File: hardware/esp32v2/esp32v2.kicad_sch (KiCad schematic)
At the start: 27 parts, among them J1 Conn_01x02, J2 Conn_01x02, J3 Conn_01x10, U1 ESP32-S3, Y2 40MHz(10ppm)

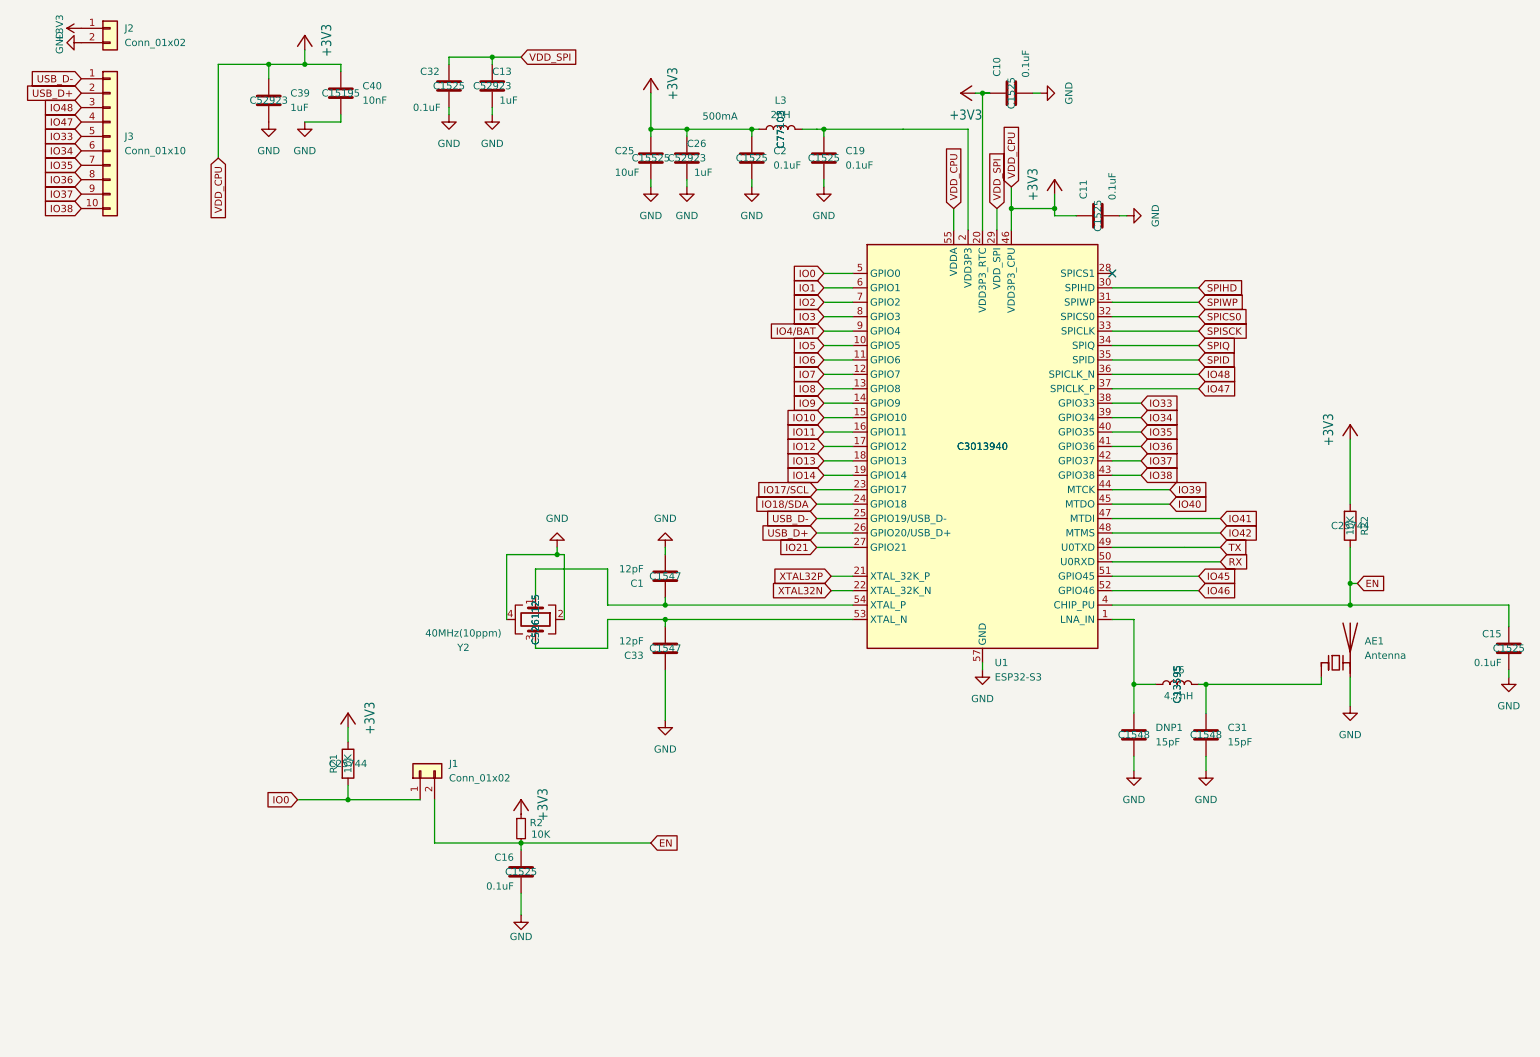
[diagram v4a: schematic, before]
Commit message: wip
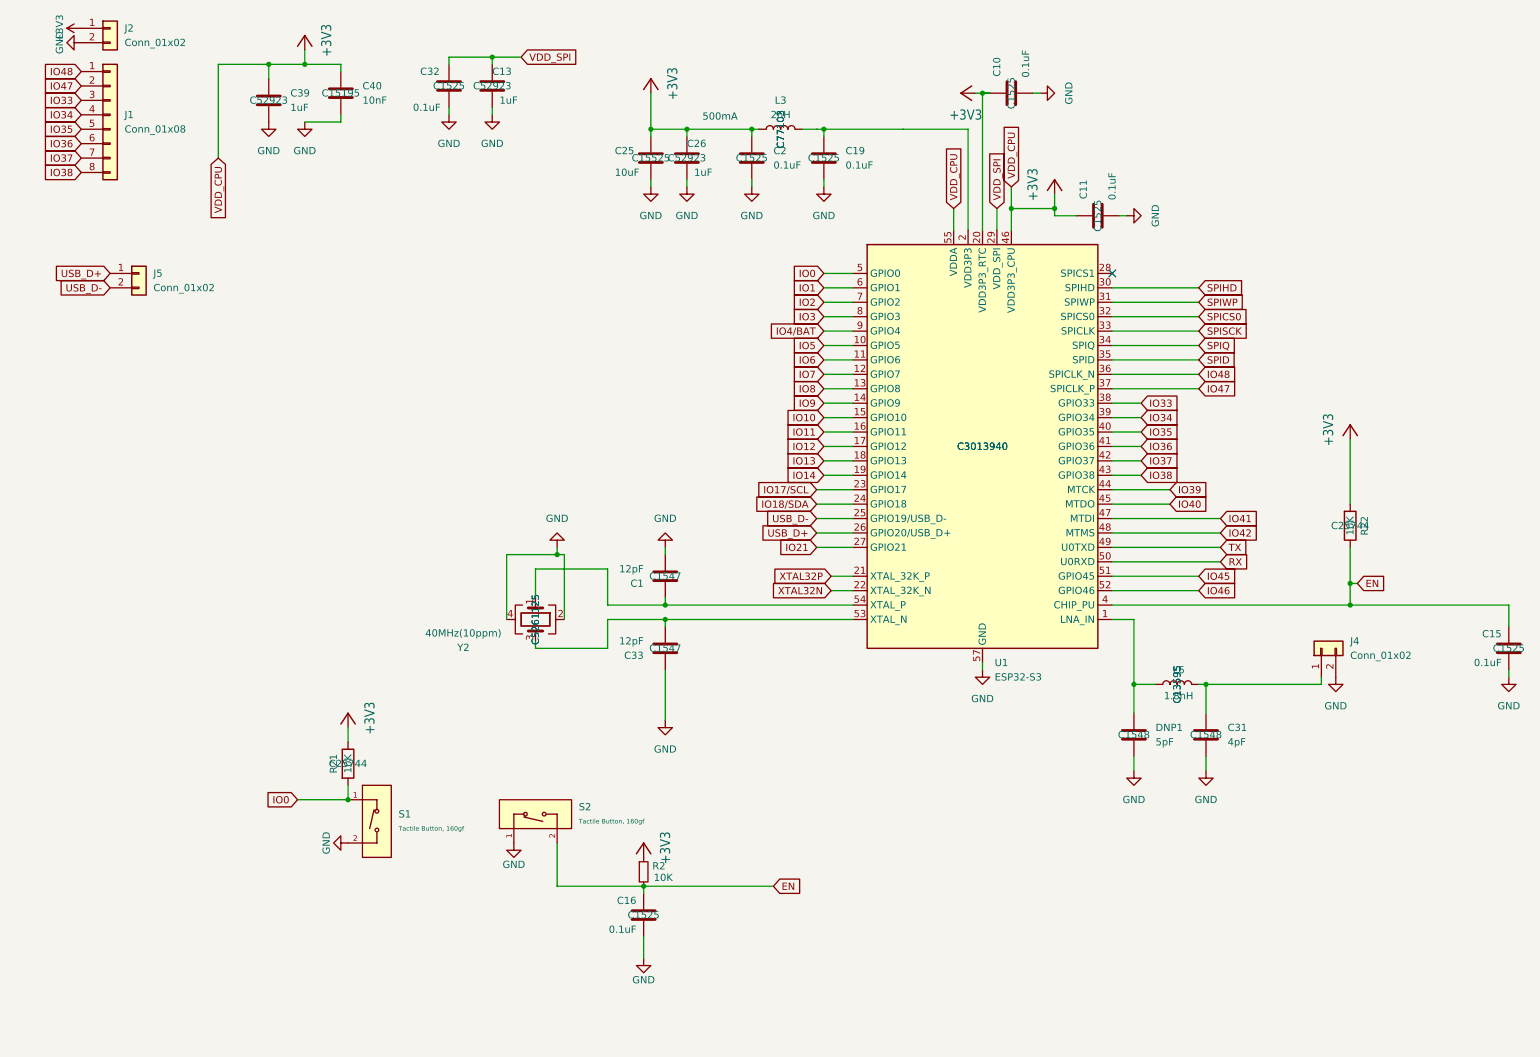
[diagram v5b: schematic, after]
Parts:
- removed AE1: Antenna, RF_Antenna:Texas_SWRA117D_2.4GHz_Left, symbol Device:Antenna_Chip
- removed J1: Conn_01x02, Connector_JST:JST_SH_BM02B-SRSS-TB_1x02-1MP_P1.00mm_Vertical, symbol Connector_Generic:Conn_01x02
- removed J3: Conn_01x10, LIB_SM10B-SRSS-TB_LF__SN_:SM10B-SRSS-TB, symbol Connector_Generic:Conn_01x10
- added J1: Conn_01x08, Connector_JST:JST_SHL_SM08B-SHLS-TF_1x08-1MP_P1.00mm_Horizontal, symbol Connector_Generic:Conn_01x08
- added J4: Conn_01x02, Connector_Coaxial:U.FL_Molex_MCRF_73412-0110_Vertical, symbol Connector_Generic:Conn_01x02
- added J5: Conn_01x02, Connector_JST:JST_SH_BM02B-SRSS-TB_1x02-1MP_P1.00mm_Vertical, symbol Connector_Generic:Conn_01x02
- added S1, S2: Tactile Button, 160gf, PCM_JLCPCB:SW_TS-1088-AR02016, symbol PCM_JLCPCB-Connectors_Buttons:Tactile Button, 160gf, 12V, 50mA, 4.0mm
- C31: value 15pF -> 4pF
- DNP1: value 15pF -> 5pF
- L6: value 4.7nH -> 1.8nH
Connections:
- net EN: now also S2.2 (B)
- net GND: now also J4.2 (Pin_2), S1.2 (B), S2.1 (A)
- net IO0: now also S1.1 (A)
- net IO33: now also J1.3 (Pin_3)
- net IO34: now also J1.4 (Pin_4)
- net IO35: now also J1.5 (Pin_5)
- net IO36: now also J1.6 (Pin_6)
- net IO37: now also J1.7 (Pin_7)
- net IO38: now also J1.8 (Pin_8)
- net IO47: now also J1.2 (Pin_2)
- net IO48: now also J1.1 (Pin_1)
- net USB_D+: now also J5.1 (Pin_1)
- net USB_D-: now also J5.2 (Pin_2)
- net at C31.1, L6.2: now also J4.1 (Pin_1)
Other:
- moved on the sheet: C16, R2
